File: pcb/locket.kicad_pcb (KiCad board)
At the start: 2 copper layers, 1 part, among them U1 ESP32-S3-WROOM-1

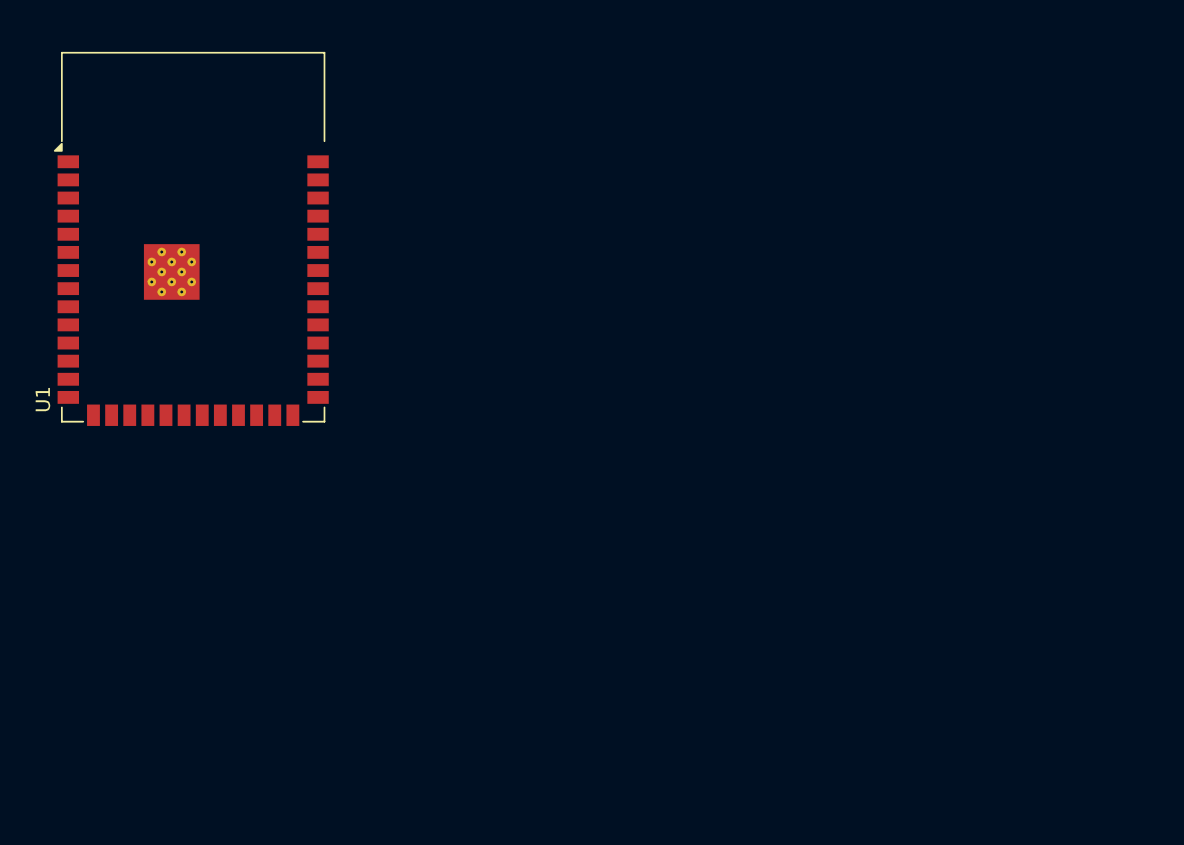
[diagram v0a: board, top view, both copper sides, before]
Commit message: schematic final and starting layout
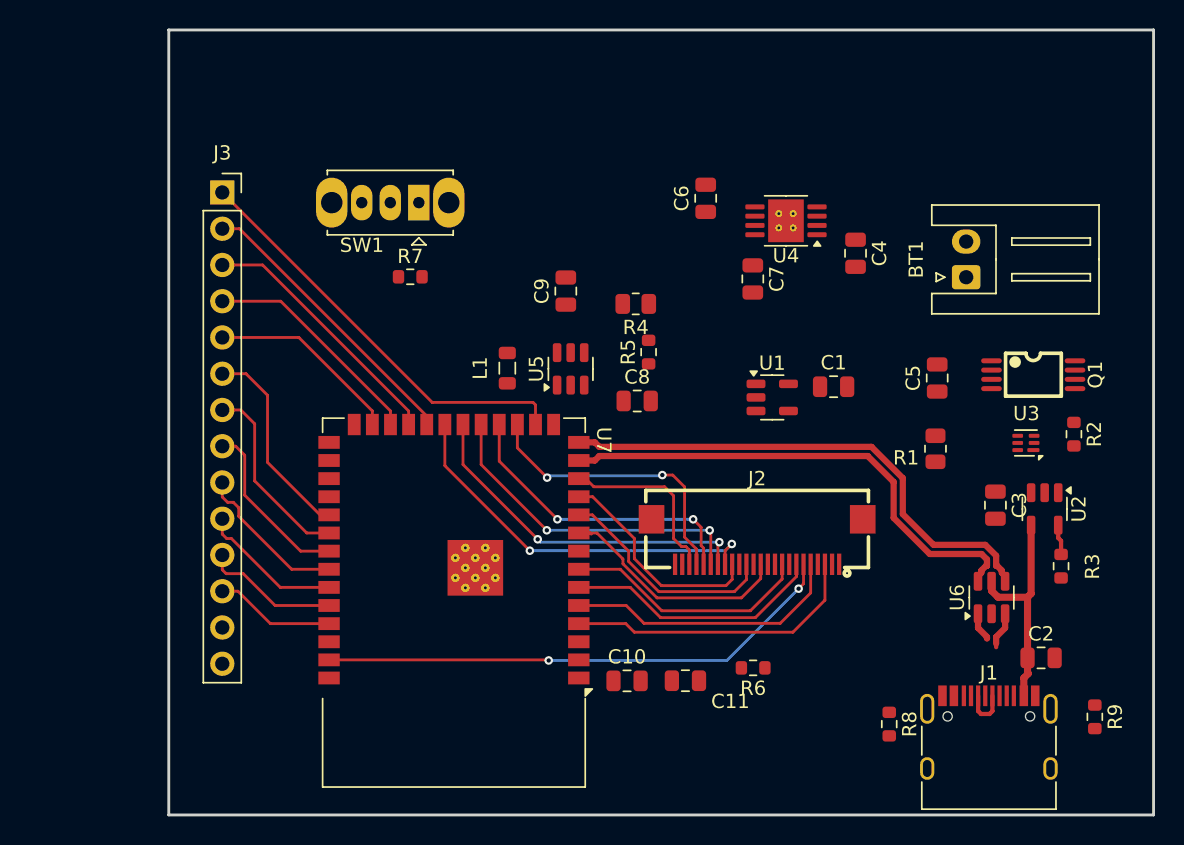
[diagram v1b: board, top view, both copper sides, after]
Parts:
- added BT1: Battery_Cell, Connector_JST:JST_XH_S2B-XH-A_1x02_P2.50mm_Horizontal, F.Cu at (169.7, 82.3)
- added C1: 2.2u, Capacitor_SMD:C_0805_2012Metric, F.Cu at (160.4, 90.0)
- added C10: 10u, Capacitor_SMD:C_0805_2012Metric, F.Cu at (145.9, 110.6)
- added C11: 2.2u, Capacitor_SMD:C_0805_2012Metric, F.Cu at (150.0, 110.6)
- added C2: 2.2u, Capacitor_SMD:C_0805_2012Metric, F.Cu at (174.9, 109.0)
- added C3: 2.2u, Capacitor_SMD:C_0805_2012Metric, F.Cu at (171.7, 98.3)
- added C4: 2.2u, Capacitor_SMD:C_0805_2012Metric, F.Cu at (161.9, 80.7)
- added C5: 0.1u, Capacitor_SMD:C_0805_2012Metric, F.Cu at (167.6, 89.4)
- added C6: 2.2u, Capacitor_SMD:C_0805_2012Metric, F.Cu at (151.4, 76.8)
- added C7: 2.2u, Capacitor_SMD:C_0805_2012Metric, F.Cu at (154.7, 82.5)
- added C8: 2.2u, Capacitor_SMD:C_0805_2012Metric, F.Cu at (146.6, 91.0)
- added C9: 2.2u, Capacitor_SMD:C_0805_2012Metric, F.Cu at (141.6, 83.3)
- added J1: USB_C_Receptacle_USB2.0_16P, Connector_USB:USB_C_Receptacle_HRO_TYPE-C-31-M-12, F.Cu at (171.2, 115.7)
- added J2: Conn_01x24_Pin, mykicadfootprints:FPC-SMD_P0.50-24P_QCHF-SM-H2.0, F.Cu at (155.0, 100.9)
- added J3: Conn_01x14_Pin, Connector_PinSocket_2.54mm:PinSocket_1x14_P2.54mm_Vertical, F.Cu at (117.5, 76.4)
- added L1: 2.2uH, Inductor_SMD:L_0805_2012Metric, F.Cu at (137.5, 88.7)
- added Q1: AO8810, mykicadfootprints:TSSOP-8_L4.4-W3.0-P0.65-LS6.4-BL, F.Cu at (174.3, 89.2)
- added R1: 300, Resistor_SMD:R_0805_2012Metric, F.Cu at (167.5, 94.3)
- added R2: 5.1k, Resistor_SMD:R_0603_1608Metric, F.Cu at (177.2, 93.3)
- added R3: 5.1k, Resistor_SMD:R_0603_1608Metric, F.Cu at (176.3, 102.6)
- added R4: 45k, Resistor_SMD:R_0805_2012Metric, F.Cu at (146.5, 84.2)
- added R5: 5.1k, Resistor_SMD:R_0603_1608Metric, F.Cu at (147.4, 87.6)
- added R6: 5.1k, Resistor_SMD:R_0603_1608Metric, F.Cu at (154.7, 109.7)
- added R7: 5.1k, Resistor_SMD:R_0603_1608Metric, F.Cu at (130.7, 82.3)
- added R8: 5.1k, Resistor_SMD:R_0603_1608Metric, F.Cu at (164.3, 113.6)
- added R9: 5.1k, Resistor_SMD:R_0603_1608Metric, F.Cu at (178.7, 113.1)
- added SW1: SW_Push, Button_Switch_THT:SW_Slide_SPDT_Straight_CK_OS102011MS2Q, F.Cu at (131.3, 77.1)
- added U2: MCP73812T-420I-OT, Package_TO_SOT_SMD:SOT-23-5, F.Cu at (175.2, 98.6)
- added U3: BQ297xy, Package_SON:WSON-6_1.5x1.5mm_P0.5mm, F.Cu at (173.8, 93.9)
- added U4: MIC5356-SGYMME, Package_SO:MSOP-8-1EP_3x3mm_P0.65mm_EP2.5x3mm_Mask1.73x2.36mm_ThermalVias, F.Cu at (157.0, 78.4)
- added U5: TLV61070ADBV, Package_TO_SOT_SMD:SOT-23-6, F.Cu at (141.9, 88.8)
- added U6: USBLC6-2SC6, Package_TO_SOT_SMD:SOT-23-6, F.Cu at (171.4, 104.8)
- added U7: ESP32-S3-WROOM-1, RF_Module:ESP32-S3-WROOM-1, F.Cu at (133.8, 105.2)
- U1: value ESP32-S3-WROOM-1 -> TLV73328PDBV; footprint RF_Module:ESP32-S3-WROOM-1 -> Package_TO_SOT_SMD:SOT-23-5
- moved U1 42.1 mm to (156.1, 90.8)
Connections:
- U1 pad 1: Net-(U1-GND-Pad1) -> +3V3
- U1 pad 2: unconnected-(U1-3V3-Pad2) -> GND
- U1 pad 3: unconnected-(U1-EN-Pad3) -> /CAM_PWR_EN
- U1 pad 4: /CAM_SIOD -> unconnected-(U1-NC-Pad4)
- U1 pad 5: /CAM_SIOC -> +1V8
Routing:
- net /CAM_RESET: track 0.00 -> 36.9 mm, vias 0 -> 2
- net /USB_D+: track 0.00 -> 36.1 mm
- net /USB_D-: track 0.00 -> 35.0 mm
- net /SD_CS: track 0.00 -> 29.5 mm
- net /CAM_PCLK: track 0.00 -> 27.3 mm, vias 0 -> 2
- net /D6: track 0.00 -> 24.6 mm, vias 0 -> 2
- net /D2: track 0.00 -> 23.1 mm, vias 0 -> 2
- net /D5: track 0.00 -> 21.3 mm, vias 0 -> 2
- net /CAM_SIOD: track 0.00 -> 20.9 mm
- net /D3: track 0.00 -> 20.4 mm, vias 0 -> 2
- net /TOUCH_INT: track 0.00 -> 20.4 mm
- net /CAM_SIOC: track 0.00 -> 19.6 mm
- net /TOUCH_SDA: track 0.00 -> 18.2 mm
- net /CAM_VSYNC: track 0.00 -> 18.2 mm
- net /CAM_HREF: track 0.00 -> 17.4 mm
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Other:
- board outline added: 69 x 55 mm
